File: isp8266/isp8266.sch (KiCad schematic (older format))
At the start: 65 parts, among them J1 Bottom, J10 BAT2, J11 USB_C_Receptacle_USB2.0, J12 F1, J2 Up, J7 F0, J8 BAT1, Q1 S8050, Q2 S8050, Q3 BSS138, Q4 IRLML6402, Q5 BSS138, Q6 IRLML6402, U1 CH340C, U2 AP1117-33, U3 IP5306, U4 ESP-12E

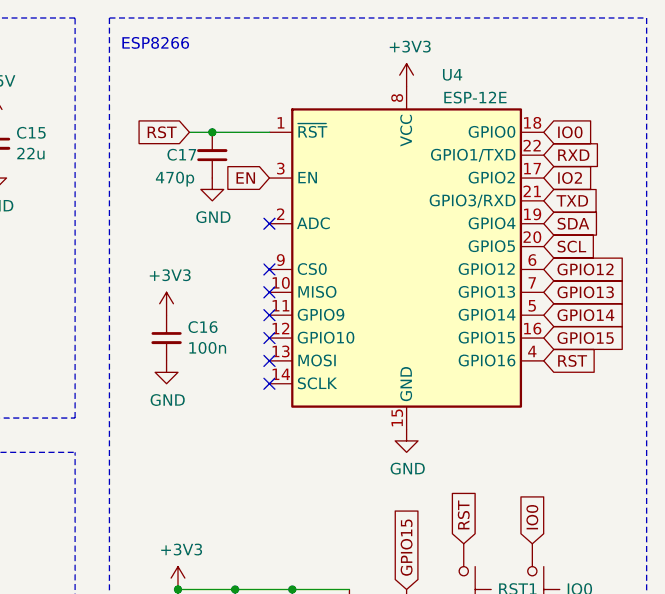
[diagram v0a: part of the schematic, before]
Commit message: Routing
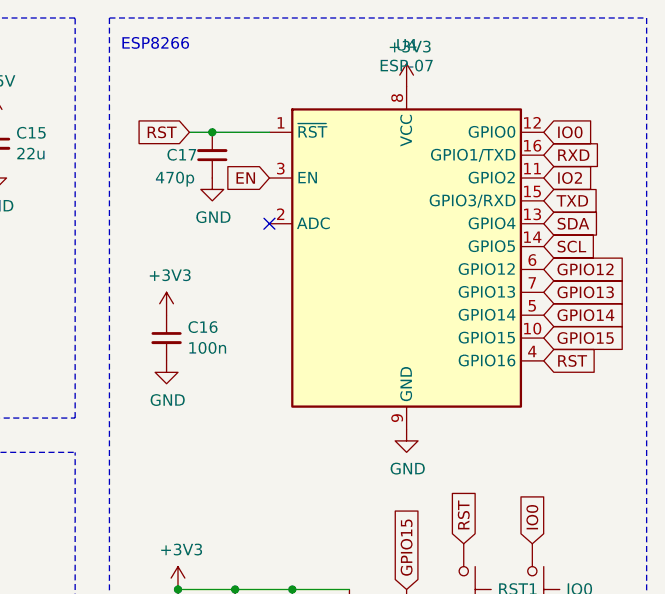
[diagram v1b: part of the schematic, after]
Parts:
- removed U4: ESP-12E, RF_Module:ESP-12E, symbol RF_Module:ESP-12E
- added U4: ESP-07, RF_Module:ESP-07, symbol RF_Module:ESP-07
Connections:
- net +3V3: now also U4.8 (VCC)
- net -BATT: now also U4.9 (GND)
- net EN: now also U4.3 (EN)
- net GPIO12: now also U4.6 (GPIO12)
- net GPIO13: now also U4.7 (GPIO13)
- net GPIO14: now also U4.5 (GPIO14)
- net GPIO15: now also U4.10 (GPIO15)
- net IO0: now also U4.12 (GPIO0)
- net IO2: now also U4.11 (GPIO2)
- net RST: now also U4.1 (~RST), U4.4 (GPIO16)
- net RXD: now also U4.16 (GPIO1/TXD)
- net SCL: now also U4.14 (GPIO5)
- net SDA: now also U4.13 (GPIO4)
- net TXD: now also U4.15 (GPIO3/RXD)
- no-connect marks 14 -> 8
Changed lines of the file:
@@
 	1    0    0    -1
 $EndComp
-NoConn ~ 8950 1700
-NoConn ~ 8950 1800
-NoConn ~ 8950 1900
-NoConn ~ 8950 2000
-NoConn ~ 8950 2100
-NoConn ~ 8950 2200
 NoConn ~ 8950 1500
 Text GLabel 10150 1500 2    50   Input ~ 0
@@
 Text GLabel 10150 1600 2    50   Input ~ 0
 SCL
-$Comp
-L RF_Module:ESP-12E U4
-U 1 1 637F3A80
-P 9550 1700
-F 0 "U4" H 9750 2550 50  0000 C CNN
-F 1 "ESP-12E" H 9850 2450 50  0000 C CNN
-F 2 "RF_Module:ESP-12E" H 9550 1700 50  0001 C CNN
-F 3 "http://wiki.ai-thinker.com/_media/esp8266/esp8266_series_modules_user_manual_v1.1.pdf" H 9200 1800 50  0001 C CNN
-	1    9550 1700
-	1    0    0    -1
-$EndComp
 Text GLabel 10150 2000 2    50   Input ~ 0
 GPIO15
@@
 $EndComp
 $Comp
-L power:+BATT #PWR?
+L power:+BATT #PWR0106
 U 1 1 63A6D1A8
 P 10000 4500
-F 0 "#PWR?" H 10000 4350 50  0001 C CNN
+F 0 "#PWR0106" H 10000 4350 50  0001 C CNN
 F 1 "+BATT" H 10015 4673 50  0000 C CNN
 F 2 "" H 10000 4500 50  0001 C CNN
@@
 	-1   0    0    1
 $EndComp
+$Comp
+L RF_Module:ESP-07 U4
+U 1 1 63A9E644
+P 9550 1700
+F 0 "U4" H 9550 2681 50  0000 C CNN
+F 1 "ESP-07" H 9550 2590 50  0000 C CNN
+F 2 "RF_Module:ESP-07" H 9550 1700 50  0001 C CNN
+F 3 "http://wiki.ai-thinker.com/_media/esp8266/esp8266_series_modules_user_manual_v1.1.pdf" H 9200 1800 50  0001 C CNN
+	1    9550 1700
+	1    0    0    -1
+$EndComp
 $EndSCHEMATC
